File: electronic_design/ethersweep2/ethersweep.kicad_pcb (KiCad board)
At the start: 2 copper layers, 60 x 60 mm, 20 parts, among them J1 Jack-DC, J2 ETH_LEFT, J3 ETH_RIGHT, J5 Conn_01x04_Female, M1 Stepper_Motor_bipolar

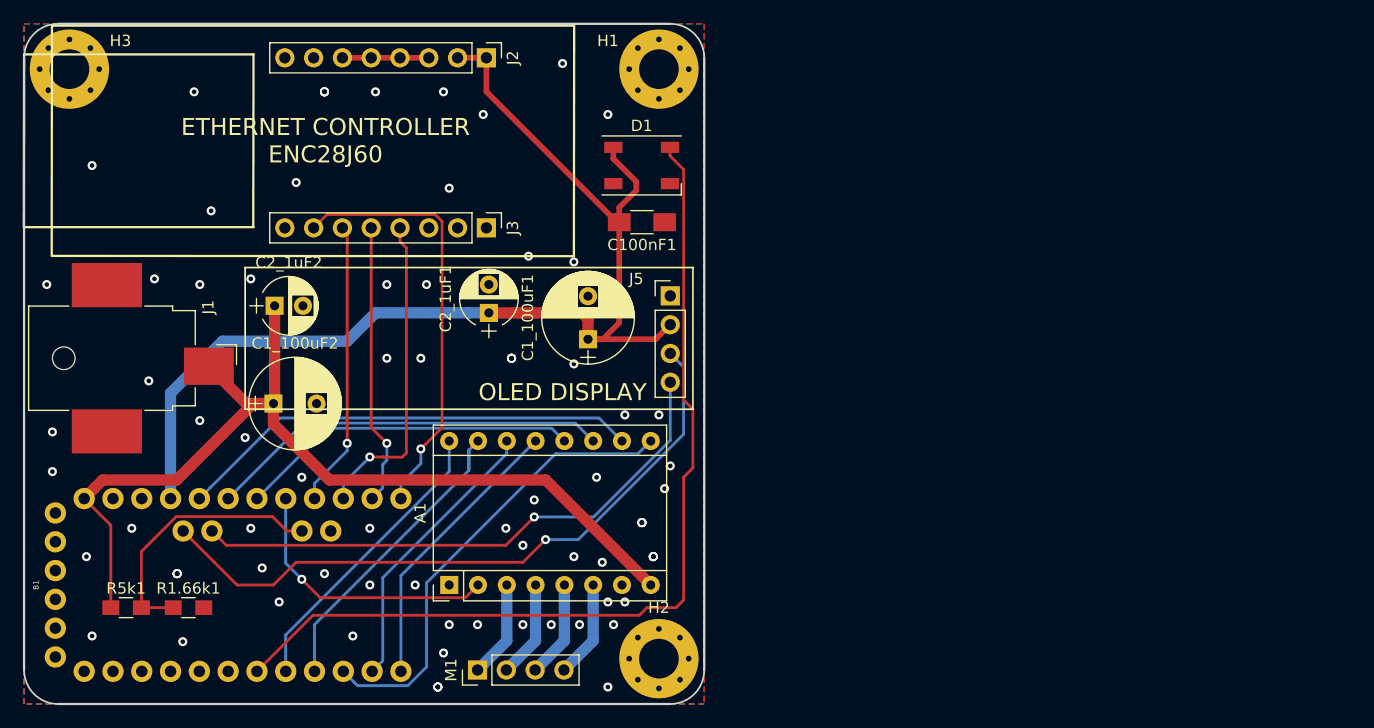
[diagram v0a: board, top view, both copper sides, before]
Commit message: raw component layout done
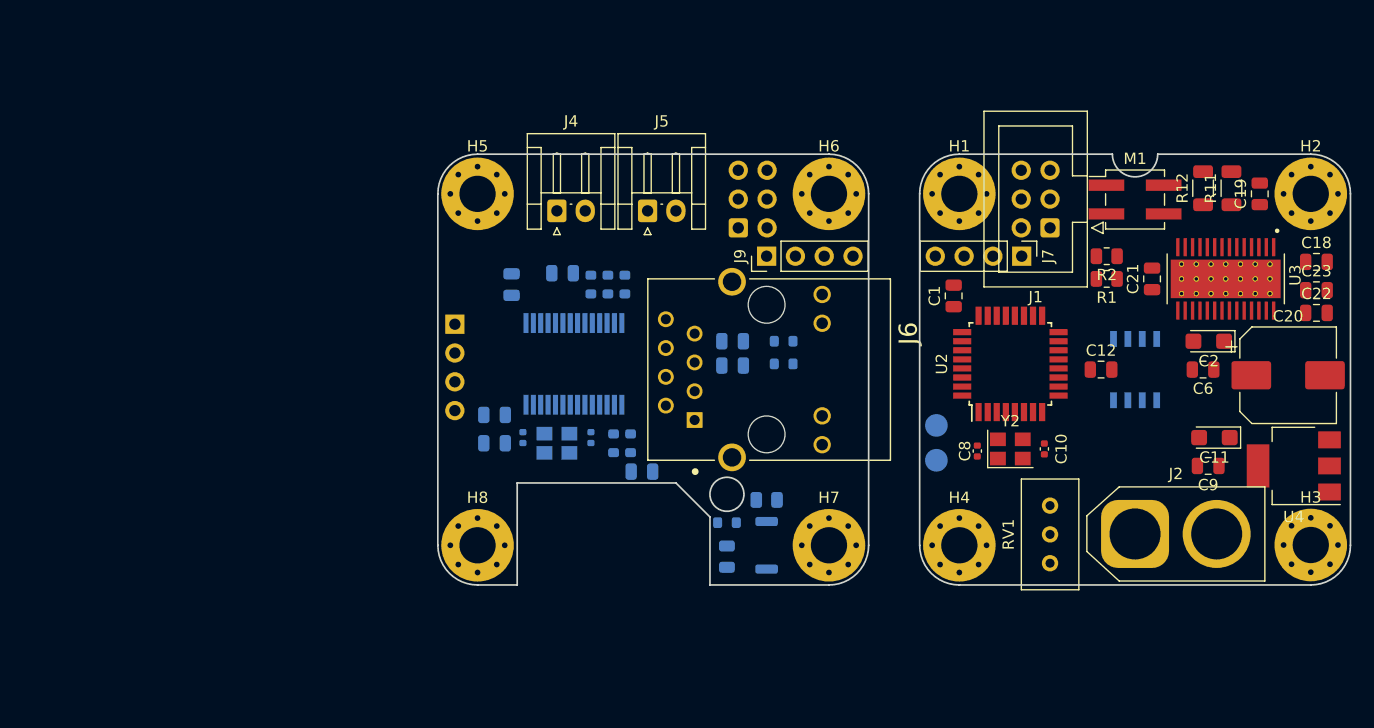
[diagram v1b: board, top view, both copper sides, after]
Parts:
- removed A1: Pololu_Breakout_DRV8825, Modules:Pololu_Breakout-16_15.2x20.3mm
- removed B1: ARDUINO_PRO_MINI, arduino_pro_mini:ARDUINO_PRO_MINI
- removed C100nF1: C, Capacitors_SMD:C_1206_HandSoldering
- removed C1_100uF1, C1_100uF2: CP, Capacitors_THT:CP_Radial_D8.0mm_P3.80mm
- removed C2_1uF1, C2_1uF2: CP, Capacitors_THT:CP_Radial_D5.0mm_P2.50mm
- removed the G*** at (110.4, 81.7)
- removed R1.66k1, R5k1: R, Resistors_SMD:R_0805_HandSoldering
- added C1: C100nF, Capacitor_SMD:C_0805_2012Metric, F.Cu at (166.5, 93.5)
- added C10: C22pF, Capacitor_SMD:C_0402_1005Metric, F.Cu at (174.5, 107.0)
- added C11: C22uF, Capacitor_Tantalum_SMD:CP_EIA-3216-12_Kemet-S, F.Cu at (189.5, 106.0)
- added C12: C100nF, Capacitor_SMD:C_0805_2012Metric, F.Cu at (179.5, 100.0)
- added C13: C1uF, Capacitor_SMD:C_0805_2012Metric, B.Cu at (127.5, 92.5)
- added C14: C1uF, Capacitor_SMD:C_0805_2012Metric, B.Cu at (139.0, 109.0)
- added C15: C1uF, Capacitor_SMD:C_0805_2012Metric, B.Cu at (132.0, 91.5)
- added C16: C1uF, Capacitor_SMD:C_0805_2012Metric, B.Cu at (147.0, 97.5)
- added C17: C1uF, Capacitor_SMD:C_0805_2012Metric, B.Cu at (147.0, 99.6)
- added C18: C10nF, Capacitor_SMD:C_0805_2012Metric, F.Cu at (198.5, 90.5)
- added C19: C100nF, Capacitor_SMD:C_0805_2012Metric, F.Cu at (193.5, 84.5)
- added C2: C22uF, Capacitor_Tantalum_SMD:CP_EIA-3216-12_Kemet-S, F.Cu at (189.0, 97.5)
- added C20: C100uF, Capacitor_SMD:CP_Elec_8x10, F.Cu at (196.0, 100.5)
- added C21: C0.47uF, Capacitor_SMD:C_0805_2012Metric, F.Cu at (184.0, 92.0)
- added C22: C100nF, Capacitor_SMD:C_0805_2012Metric, F.Cu at (198.5, 95.0)
- added C23: C100nF, Capacitor_SMD:C_0805_2012Metric, F.Cu at (198.5, 93.0)
- added C3: C1uF, Capacitor_SMD:C_0805_2012Metric, B.Cu at (126.0, 106.5)
- added C4: C22pF, Capacitor_SMD:C_0402_1005Metric, B.Cu at (134.5, 106.0)
- added C5: C22pF, Capacitor_SMD:C_0402_1005Metric, B.Cu at (128.5, 106.0)
- added C6: C100nF, Capacitor_SMD:C_0805_2012Metric, F.Cu at (188.5, 100.0)
- added C7: C1uF, Capacitor_SMD:C_0805_2012Metric, B.Cu at (126.0, 104.0)
- added C8: C22pF, Capacitor_SMD:C_0402_1005Metric, F.Cu at (168.6, 107.2)
- added C9: C100nF, Capacitor_SMD:C_0805_2012Metric, F.Cu at (188.9, 108.5)
- added H4: MountingHole_Pad, MountingHole:MountingHole_3.2mm_M3_Pad_Via, F.Cu at (167.0, 115.5)
- added H5: MountingHole_Pad, MountingHole:MountingHole_3.2mm_M3_Pad_Via, F.Cu at (124.5, 84.5)
- added H6: MountingHole_Pad, MountingHole:MountingHole_3.2mm_M3_Pad_Via, F.Cu at (155.5, 84.5)
- added H7: MountingHole_Pad, MountingHole:MountingHole_3.2mm_M3_Pad_Via, F.Cu at (155.5, 115.5)
- added H8: MountingHole_Pad, MountingHole:MountingHole_3.2mm_M3_Pad_Via, F.Cu at (124.5, 115.5)
- added J4: Conn_01x02_Male, Connector_JST:JST_EH_S2B-EH_1x02_P2.50mm_Horizontal, F.Cu at (131.5, 86.0)
- added J6: HR911105A, modules:HANRUN_HR911105A, F.Cu at (150.0, 100.0)
- added J7: Conn_01x04_Female, Connector_PinHeader_2.54mm:PinHeader_1x04_P2.54mm_Vertical, F.Cu at (172.5, 90.0)
- added J8: AVR-ISP-6, Connector_IDC:IDC-Header_2x03_P2.54mm_Vertical, B.Cu at (147.5, 87.5)
- added J9: Conn_01x04_Female, Connector_PinHeader_2.54mm:PinHeader_1x04_P2.54mm_Vertical, F.Cu at (150.0, 90.0)
- added R1: R5k, Resistor_SMD:R_0805_2012Metric, F.Cu at (180.0, 92.0)
- added R10: R1k, Resistor_SMD:R_0603_1608Metric, B.Cu at (136.0, 92.5)
- added R11: R200mOHM, Resistor_SMD:R_1206_3216Metric, F.Cu at (191.0, 84.0)
- added R12: R200mOHM, Resistor_SMD:R_1206_3216Metric, F.Cu at (188.5, 84.0)
- added R13: R330, Resistor_SMD:R_0603_1608Metric, B.Cu at (146.5, 113.5)
- added R2: R5k, Resistor_SMD:R_0805_2012Metric, F.Cu at (180.0, 90.0)
- added R3: R10k, Resistor_SMD:R_0805_2012Metric, B.Cu at (150.0, 111.5)
- added R4: R1k, Resistor_SMD:R_0603_1608Metric, B.Cu at (137.5, 92.5)
- added R5: R330, Resistor_SMD:R_0603_1608Metric, B.Cu at (151.5, 97.5)
- added R6: R330, Resistor_SMD:R_0603_1608Metric, B.Cu at (151.5, 99.5)
- added R7: R1k, Resistor_SMD:R_0603_1608Metric, B.Cu at (138.0, 106.5)
- added R8: R1k, Resistor_SMD:R_0603_1608Metric, B.Cu at (136.5, 106.5)
- added R9: R1k, Resistor_SMD:R_0603_1608Metric, B.Cu at (134.5, 92.5)
- added RV1: R_POT_10K, Potentiometer_THT:Potentiometer_Bourns_3296W_Vertical, F.Cu at (175.0, 112.0)
- added RX1: TestPoint, TestPoint:TestPoint_Pad_D2.0mm, B.Cu at (165.0, 108.0)
- added SW1: SW_Push, Button_Switch_SMD:SW_Push_SPST_NO_Alps_SKRK, B.Cu at (150.0, 115.5)
- added TX1: TestPoint, TestPoint:TestPoint_Pad_D2.0mm, B.Cu at (165.0, 104.9)
- added U1: ENC28J60x-SS, Package_SO:SSOP-28_5.3x10.2mm_P0.65mm, B.Cu at (133.0, 99.5)
- added U2: ATmega328-AU, Package_QFP:TQFP-32_7x7mm_P0.8mm, F.Cu at (171.5, 99.5)
- added U3: DRV8825PWPR, modules:IC_TPS61196PWPRQ1, F.Cu at (190.5, 92.0)
- added U4: AMS1117-3.3, Package_TO_SOT_SMD:SOT-223-3_TabPin2, F.Cu at (196.5, 108.5)
- added U5: AS5600, modules:AS5600, B.Cu at (182.5, 100.0)
- added Y1: Crystal_25MHz, Crystal:Crystal_SMD_3225-4Pin_3.2x2.5mm, B.Cu at (131.5, 106.5)
- added Y2: Crystal_8MHz, Crystal:Crystal_SMD_3225-4Pin_3.2x2.5mm, F.Cu at (171.5, 107.0)
- D1: value WS2812B -> LED; footprint LEDs:LED_WS2812B-PLCC4 -> LED_SMD:LED_0805_2012Metric; moved to B.Cu
- H1, H2, H3: value Mount -> MountingHole_Pad; footprint Mounting_Holes:MountingHole_3.5mm_Pad_Via -> MountingHole:MountingHole_3.2mm_M3_Pad_Via
- J1: value Jack-DC -> AVR-ISP-6; footprint Connectors:Barrel_Jack_CUI_PJ-036AH-SMT -> Connector_IDC:IDC-Header_2x03_P2.54mm_Vertical
- J2: value ETH_LEFT -> Conn_01x02_Male; footprint Pin_Headers:Pin_Header_Straight_1x08_Pitch2.54mm -> Connector_AMASS:AMASS_XT60-M_1x02_P7.20mm_Vertical
- J3: value ETH_RIGHT -> Conn_01x04_Female; footprint Pin_Headers:Pin_Header_Straight_1x08_Pitch2.54mm -> Connector_PinHeader_2.54mm:PinHeader_1x04_P2.54mm_Vertical; moved to B.Cu
- J5: value Conn_01x04_Female -> Conn_01x02_Male; footprint Pin_Headers:Pin_Header_Straight_1x04_Pitch2.54mm -> Connector_JST:JST_EH_S2B-EH_1x02_P2.50mm_Horizontal
- M1: footprint Pin_Headers:Pin_Header_Straight_1x04_Pitch2.54mm -> Connector_PinHeader_2.54mm:PinHeader_2x02_P2.54mm_Vertical_SMD
- moved H3 117.3 mm to (198.0, 115.5)
- moved J1 80.8 mm to (175.0, 87.5), turned to 180 degrees
- moved M1 71.3 mm to (182.5, 85.0), turned to 0 degrees
- moved J2 71.0 mm to (182.5, 114.5), turned to 0 degrees
- moved H2 70.6 mm to (198.0, 84.5)
- moved D1 35.3 mm to (146.5, 116.5), turned to 90 degrees
- moved H1 28.7 mm to (167.0, 84.5)
- moved J3 8.94 mm to (122.5, 96.0), turned to 180 degrees
- moved J5 7.76 mm to (139.5, 86.0)
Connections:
- D1 pad 1: +5V -> GND
- J1 pad 1: VCC -> MISO
- J1 pad 2: GND -> +3V3
- J1 pad 3: (no net) -> SCK
- J2 pad 1: +5V -> +12V
- J2 pad 2: +5V -> GND
- J3 pad 1: Net-(J3-Pad1) -> GND
- J3 pad 2: Net-(J3-Pad2) -> +3V3
- J3 pad 3: Net-(J3-Pad3) -> SCL
- J3 pad 4: Net-(B1-Pad15) -> SDA
- J5 pad 2: +5V -> ENDSTOP
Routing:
- net +5V: track 101.2 -> 0.00 mm
- net VCC: track 87.5 -> 0.00 mm
- net Net-(B1-Pad7): track 81.4 -> 0.00 mm
- net SCL: track 59.2 -> 0.00 mm, vias 1 -> 0
- net SDA: track 49.9 -> 0.00 mm, vias 1 -> 0
- net analog3: track 41.1 -> 0.00 mm
- net Net-(A1-Pad9): track 40.9 -> 0.00 mm
- net Net-(B1-Pad13): track 38.0 -> 0.00 mm, vias 1 -> 0
- net analog2: track 35.6 -> 0.00 mm
- net analog1: track 30.2 -> 0.00 mm
- net Net-(B1-Pad15): track 28.1 -> 0.00 mm, vias 1 -> 0
- net Net-(A1-Pad15): track 28.0 -> 0.00 mm
- net Net-(A1-Pad16): track 26.3 -> 0.00 mm
- net Net-(A1-Pad14): track 25.2 -> 0.00 mm
- net Net-(B1-Pad16): track 25.2 -> 0.00 mm, vias 1 -> 0
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- removed copper zone on B.Cu, net GND
- removed copper zone on F.Cu, net GND
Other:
- board size 60 x 60 mm -> 80.5 x 38 mm
- board text removed: "2020.02.23"
- board text removed: "ETHERNET CONTROLLER ENC28J60"
- board text removed: "OLED DISPLAY"
- board text removed: "github.com/neumi/ethersweep"
